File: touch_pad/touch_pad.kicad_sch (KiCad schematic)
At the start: 17 parts, among them J1 I/O connector, U1 HT7550-1, U2 TLV6001UIDBVR

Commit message: Complete
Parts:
- J1: footprint cycfi_library:pin_header_1x3p_2.54mm_smd_horizontal -> Connector_PinHeader_2.54mm:PinHeader_1x03_P2.54mm_Vertical_SMD_Pin1Left; LCSC (none) -> C2883760
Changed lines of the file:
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@@
     (property "Reference" "J1" (id 0) (at 172.085 49.53 0))
     (property "Value" "I/O connector" (id 1) (at 168.275 43.1769 0))
-    (property "Footprint" "cycfi_library:pin_header_1x3p_2.54mm_smd_horizontal" (id 2) (at 168.275 49.53 0)
+    (property "Footprint" "Connector_PinHeader_2.54mm:PinHeader_1x03_P2.54mm_Vertical_SMD_Pin1Left" (id 2) (at 168.275 49.53 0)
       (effects (font (size 1.27 1.27)) hide)
     )
     (property "Datasheet" "" (id 3) (at 168.275 49.53 0)
       (effects (font (size 1.27 1.27)) hide)
+    )
+    (property "LCSC" "C2883760" (id 4) (at 168.275 49.53 0)
+      (effects (font (size 1.524 1.524)) hide)
     )
     (pin "1")
@@
     )
     (path "/cd61a421-8b7f-4ccf-a635-570d47a12576"
-      (reference "J1") (unit 1) (value "I/O connector") (footprint "cycfi_library:pin_header_1x3p_2.54mm_smd_horizontal")
+      (reference "J1") (unit 1) (value "I/O connector") (footprint "Connector_PinHeader_2.54mm:PinHeader_1x03_P2.54mm_Vertical_SMD_Pin1Left")
     )
     (path "/70f433c8-6a5b-4e60-a793-4584fa8ceffe"

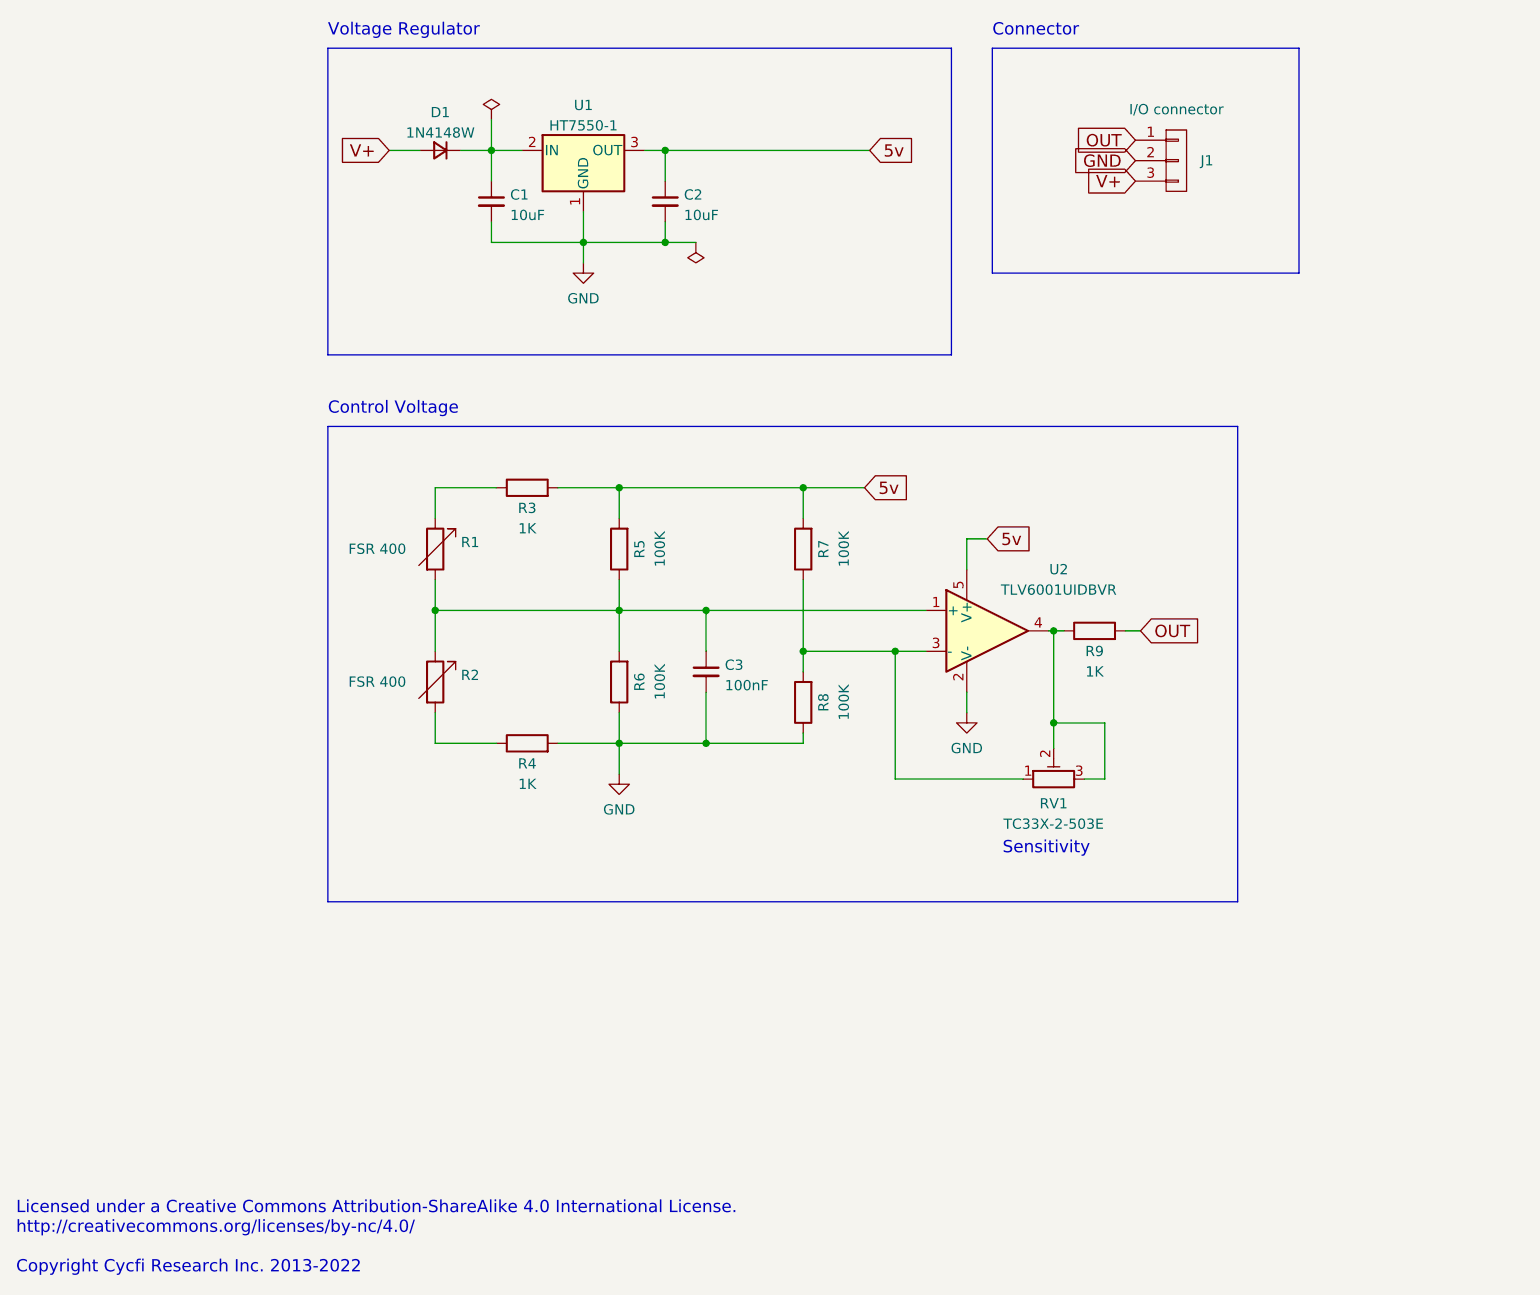
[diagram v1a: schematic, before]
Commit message: Minor tweaks
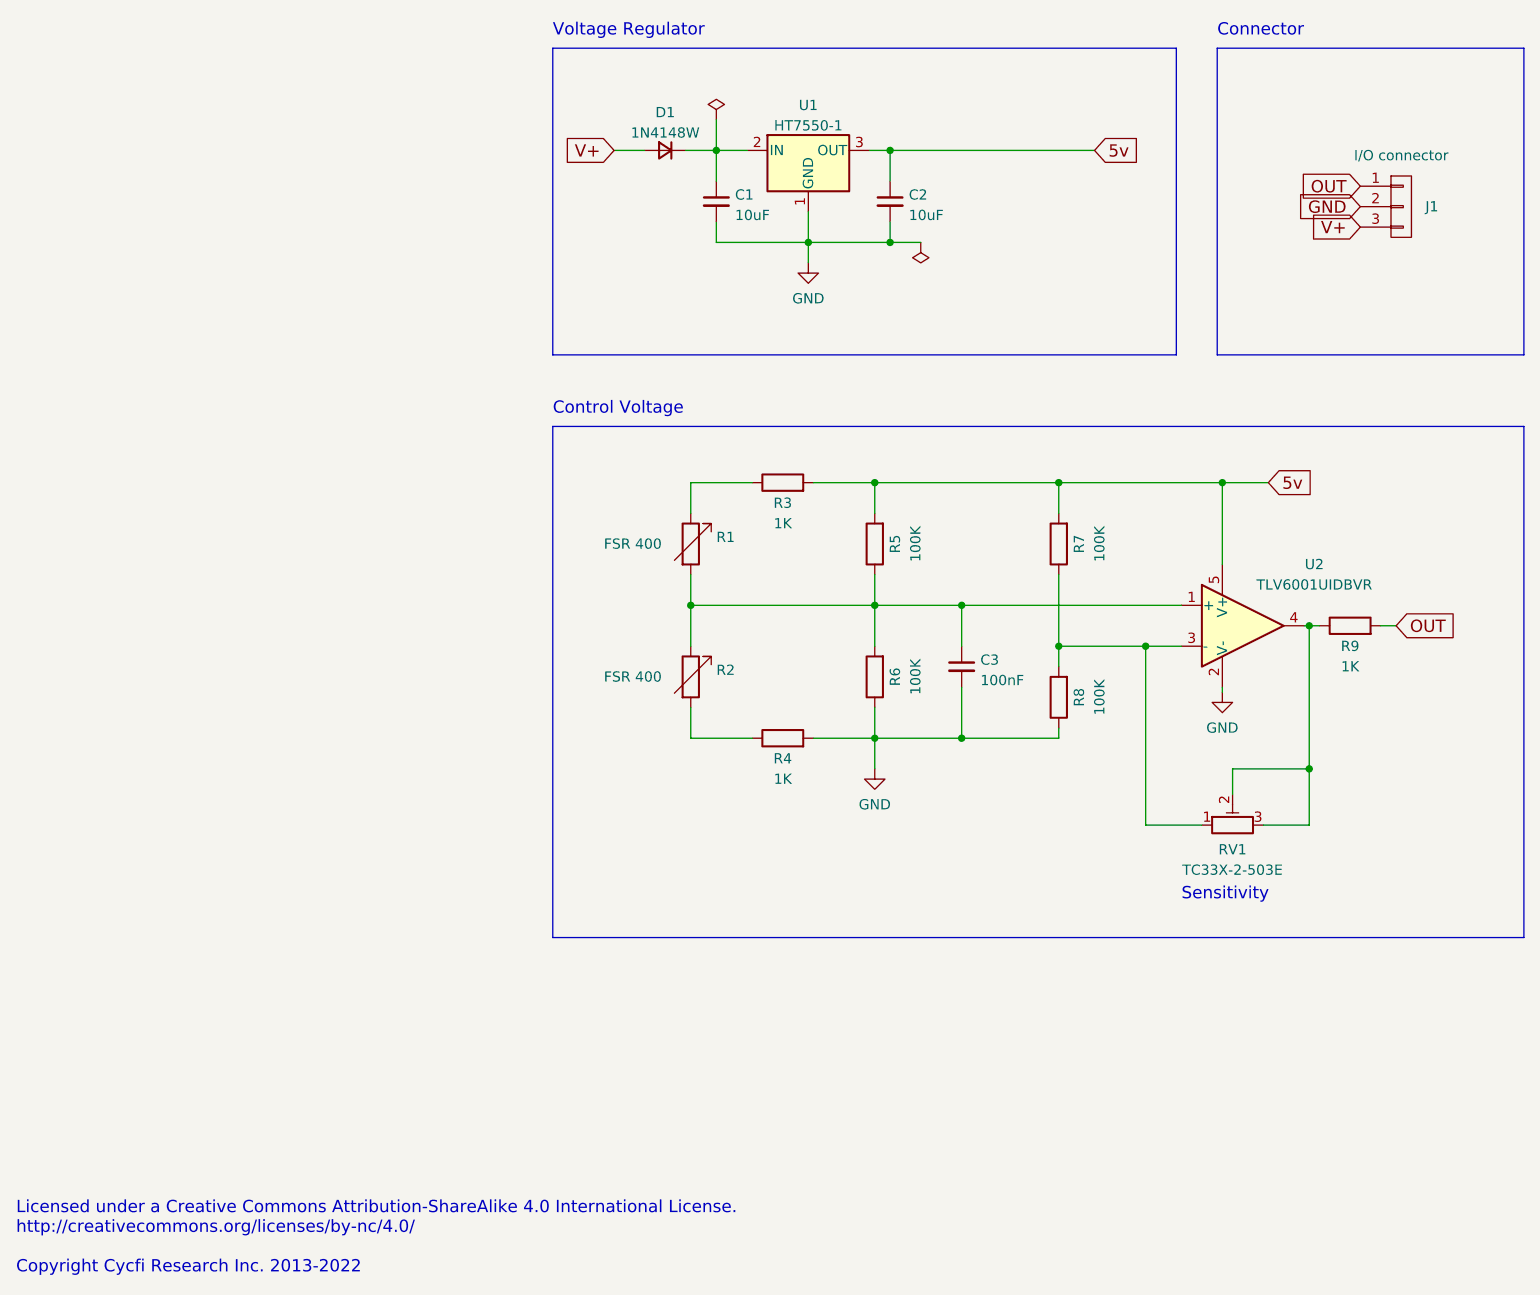
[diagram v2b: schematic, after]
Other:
- moved on the sheet: C1, C2, C3, D1, J1, R1, R2, R3, R4, R5, R6, R7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

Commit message: fabricating the touch_pad prototype
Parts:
- J1: JLCPCB_CORRECTION (none) -> 0;0;270
- U1, U2: JLCPCB_CORRECTION (none) -> 0;0;180
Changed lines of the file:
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@@
       (effects (font (size 1.524 1.524)) hide)
+    )
+    (property "JLCPCB_CORRECTION" "0;0;180" (id 5) (at 122.555 48.26 0)
+      (effects (font (size 1.27 1.27)) hide)
     )
     (pin "1")
@@
     )
     (property "LCSC" "C2883760" (id 4) (at 196.215 55.245 0)
+      (effects (font (size 1.524 1.524)) hide)
+    )
+    (property "JLCPCB_CORRECTION" "0;0;270" (id 5) (at 196.215 55.245 0)
       (effects (font (size 1.524 1.524)) hide)
     )
@@
       (effects (font (size 1.524 1.524)) hide)
     )
+    (property "JLCPCB_CORRECTION" "0;0;180" (id 5) (at 176.53 107.315 0)
+      (effects (font (size 1.27 1.27)) hide)
+    )
     (pin "2")
